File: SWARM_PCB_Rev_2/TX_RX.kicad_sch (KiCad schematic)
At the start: 86 parts

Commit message: Updated Via size to 0.25mm and ReExported Files
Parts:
- dC1, dC10, dC11, dC12, dC13, dC14, dC15, dC16, dC17, dC18, dC19, dC2, dC20, dC21, dC22, dC23, dC24, dC25, dC26, dC27, dC28, dC29, dC3, dC30, dC31, dC32, dC4, dC5, dC6, dC7, dC8, dC9: Manufacturer Murata -> (none)
- dJ1, dJ2: Manufacturer JST -> (none)
- dQ1, dQ2, dQ3, dQ4: Manufacturer Infineon Technologies -> (none)
- dR1, dR10, dR11, dR12, dR13, dR14, dR15, dR16, dR18, dR19, dR2, dR20, dR21, dR22, dR23, dR24, dR25, dR26, dR27, dR28, dR29, dR3, dR30, dR31, dR32, dR33, dR34, dR35, dR36, dR4, dR5, dR6, dR7, dR8, dR9: Manufacturer Yageo -> (none)
- dR17: Manufacturer Vishay -> (none)
- dU1, dU2: Manufacturer Texas Instruments -> (none); Package SOIC-8 Texas Instruments -> (none)
- dU3, dU4, dU8: Manufacturer Texas Instruments -> (none)
- dU5: Manufacturer Analog Devices -> (none)
- dU6: Availability In Stock -> (none); Package SC70-3 Texas Instruments -> (none); Price None -> (none)
- dU7: Availability In Stock -> (none); Manufacturer Texas Instruments -> (none); Package SOIC-8 Texas Instruments -> (none); Price None -> (none)

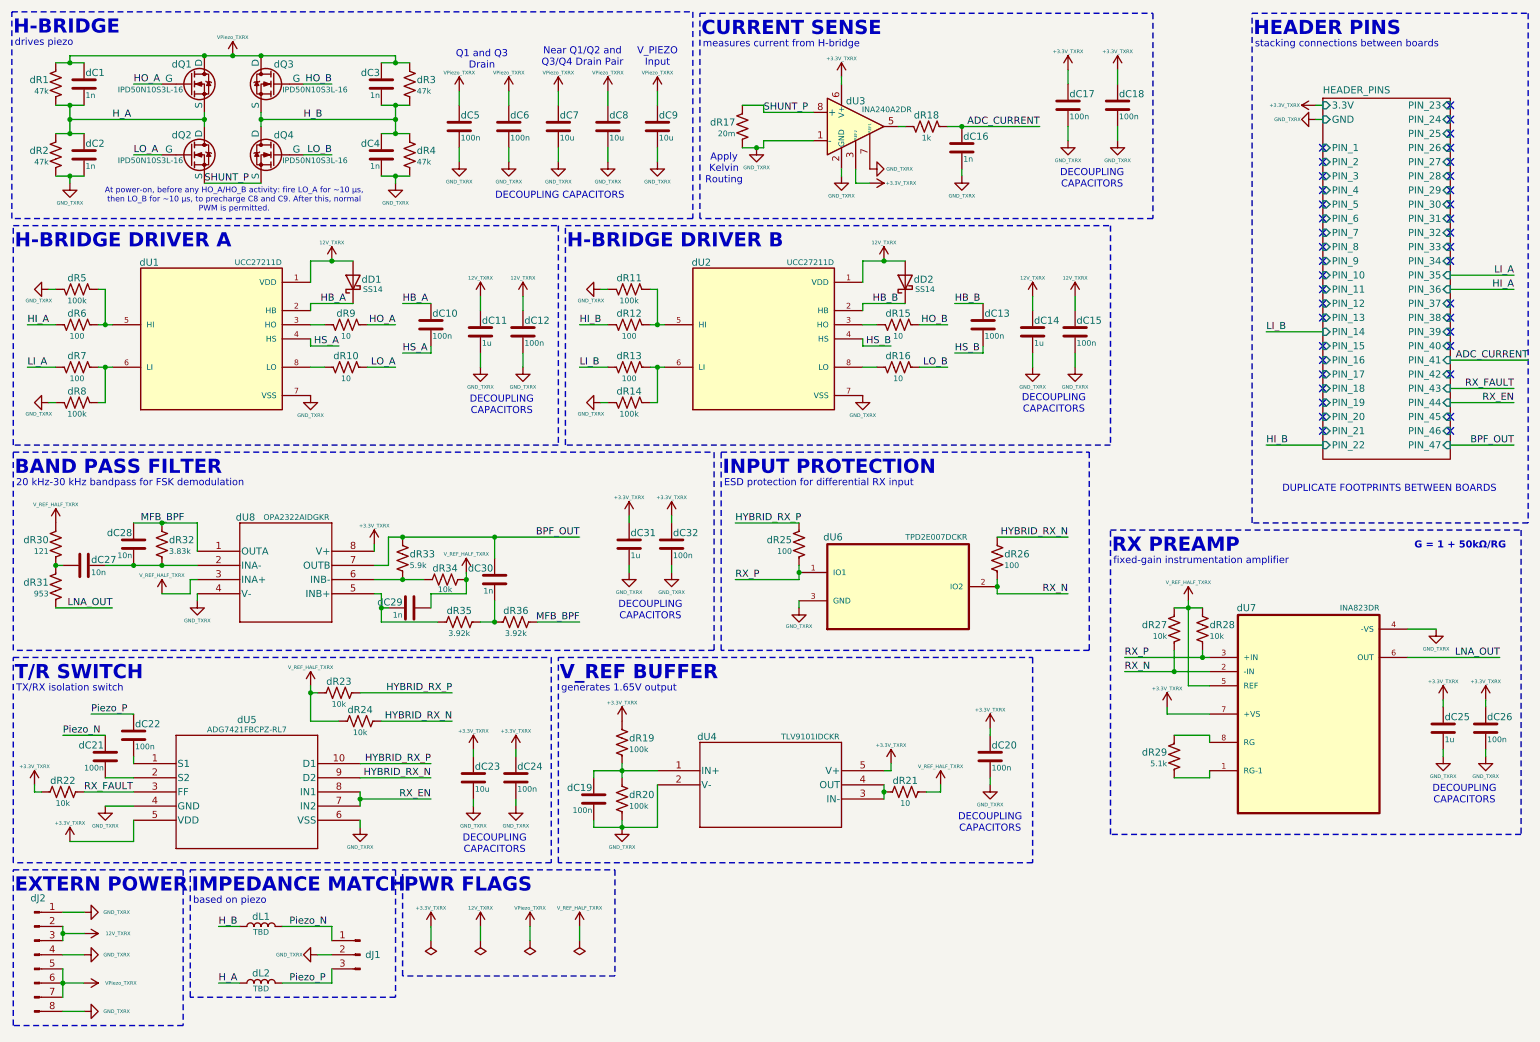
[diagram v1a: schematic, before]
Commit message: Cleaned up Schematic and Exported
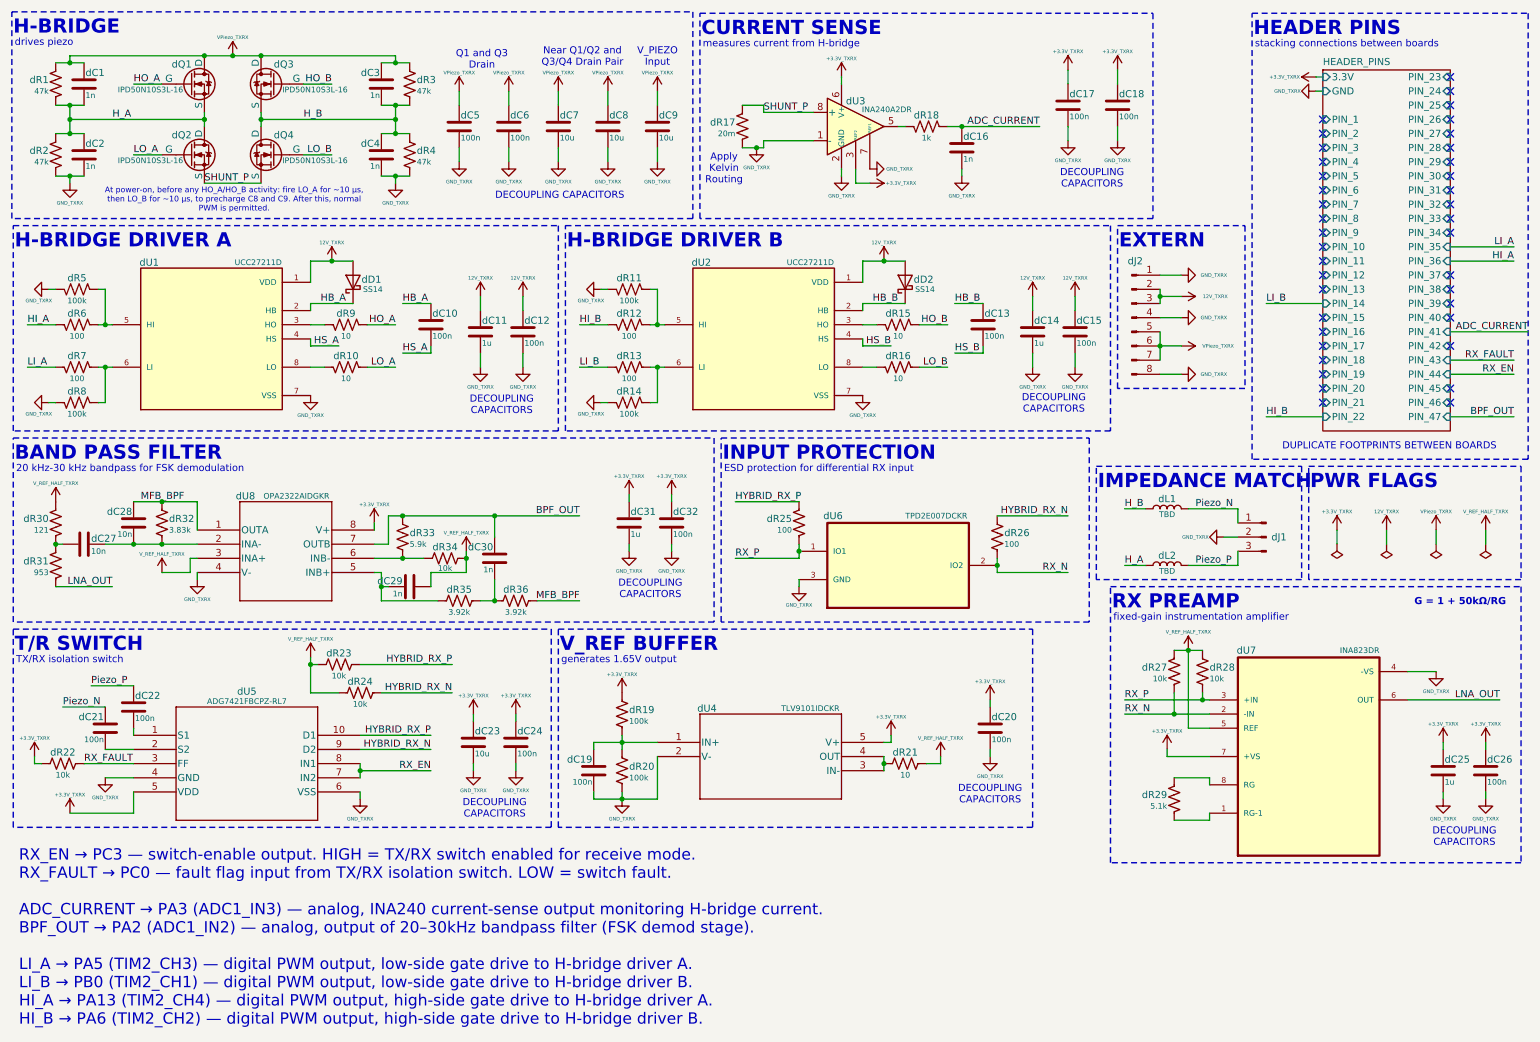
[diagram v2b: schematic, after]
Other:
- note added: "EXTERN"
- note added: "RX_EN → PC3 — switch-enable output. HIGH = TX/RX switch enabled for receive mode. RX_FAULT → PC0 — fault flag input from TX/RX isolation switch. LOW = switch fault. ADC_CURRENT → PA3 (ADC1_IN3) — analog, INA240 current-sense output monitoring H-bridge current. BPF_OUT → PA2 (ADC1_IN2) — analog, output of 20–30kHz bandpass filter (FSK demod stage). LI_A → PA5 (TIM2_CH3) — digital PWM output, low-s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"
- note removed: "EXTERN POWER"
- note removed: "based on piezo"
- moved on the sheet: dC19, dC20, dC21, dC22, dC23, dC24, dC25, dC26, dC27, dC28, dC29, dC30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
